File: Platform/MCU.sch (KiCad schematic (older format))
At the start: 34 parts, among them J10 Conn_01x05, J11 Aardvark Header SPI, J12 Aardvark Header I2C, J13 ESP8266_CONN, J14 Aardvark Header I2C, J4 Conn_01x05, J6 Debug Hdr, J7 Conn_01x05, U3 ATSAMD21E16B-M

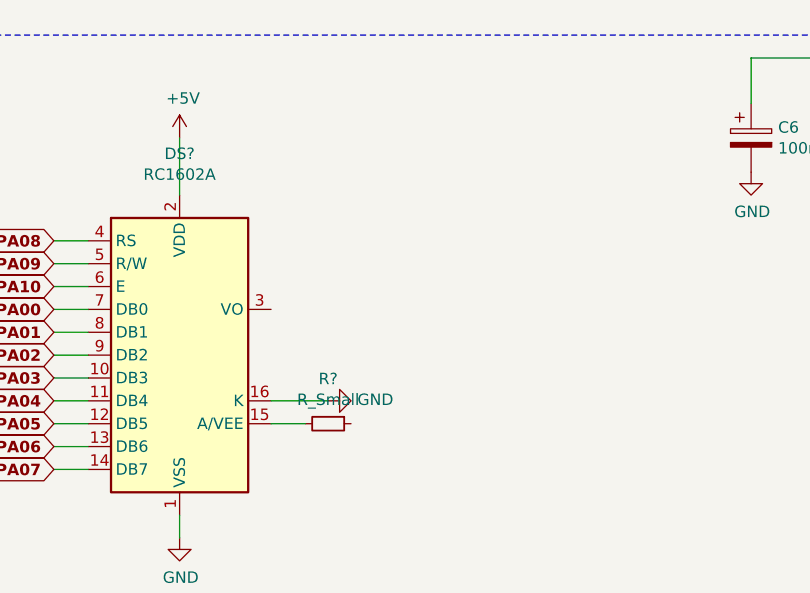
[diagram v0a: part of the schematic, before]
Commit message: Updated the schematic.
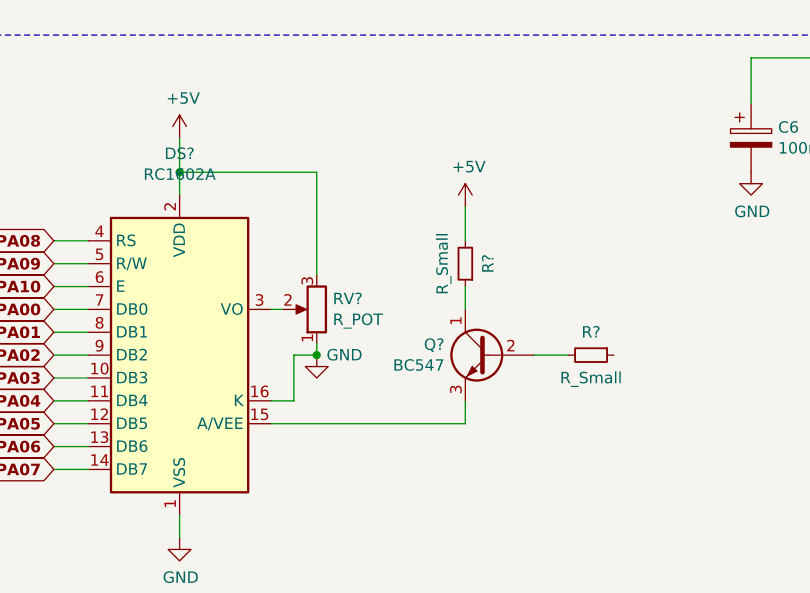
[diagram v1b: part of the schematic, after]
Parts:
- added Q?: BC547, Package_TO_SOT_THT:TO-92_Inline, symbol Transistor_BJT:BC547
- added R?: R_Small, symbol Device:R_Small
- added RV?: R_POT, symbol Device:R_POT
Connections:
- net +5V: now also R?.2, RV?.3
- net GND: now also RV?.1
- net at DS?.15 (A/VEE): now also Q?.3 (E); no longer R?.2
- net at DS?.3 (VO): now also RV?.2
- new net: Q?.1 (C), R?.1
- new net: Q?.2 (B), R?.2
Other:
- moved on the sheet: R?
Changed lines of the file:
@@
 	1750 3150 1750 3050
 Wire Wire Line
-	1750 1400 1750 1650
+	1750 1400 1750 1550
 Text GLabel 1200 1850 0    50   BiDi ~ 10
 PA08
@@
 L Device:R_Small R?
 U 1 1 6020D43B
-P 2400 2650
-F 0 "R?" V 2204 2650 50  0000 C CNN
-F 1 "R_Small" V 2295 2650 50  0000 C CNN
-F 2 "" H 2400 2650 50  0001 C CNN
-F 3 "~" H 2400 2650 50  0001 C CNN
-	1    2400 2650
+P 3550 2350
+F 0 "R?" V 3450 2350 50  0000 C CNN
+F 1 "R_Small" V 3650 2350 50  0000 C CNN
+F 2 "" H 3550 2350 50  0001 C CNN
+F 3 "~" H 3550 2350 50  0001 C CNN
+	1    3550 2350
 	0    1    1    0
 $EndComp
@@
 L power:GND #PWR?
 U 1 1 60207B70
-P 2400 2550
-F 0 "#PWR?" H 2400 2300 50  0001 C CNN
-F 1 "GND" V 2405 2422 50  0000 R CNN
-F 2 "" H 2400 2550 50  0001 C CNN
-F 3 "" H 2400 2550 50  0001 C CNN
-	1    2400 2550
-	0    -1   -1   0
+P 2350 2350
+F 0 "#PWR?" H 2350 2100 50  0001 C CNN
+F 1 "GND" H 2550 2350 50  0000 R CNN
+F 2 "" H 2350 2350 50  0001 C CNN
+F 3 "" H 2350 2350 50  0001 C CNN
+	1    2350 2350
+	1    0    0    -1
+$EndComp
+$Comp
+L power:+5V #PWR?
+U 1 1 601A2CF8
+P 3000 1700
+F 0 "#PWR?" H 3000 1550 50  0001 C CNN
+F 1 "+5V" H 3015 1873 50  0000 C CNN
+F 2 "" H 3000 1700 50  0001 C CNN
+F 3 "" H 3000 1700 50  0001 C CNN
+	1    3000 1700
+	1    0    0    -1
+$EndComp
+$Comp
+L Device:R_POT RV?
+U 1 1 601A87D3
+P 2350 2150
+F 0 "RV?" H 2280 2104 50  0000 R CNN
+F 1 "R_POT" H 2280 2195 50  0000 R CNN
+F 2 "" H 2350 2150 50  0001 C CNN
+F 3 "~" H 2350 2150 50  0001 C CNN
+	1    2350 2150
+	-1   0    0    1
 $EndComp
 Wire Wire Line
-	2150 2550 2400 2550
+	2200 2150 2150 2150
 Wire Wire Line
-	2300 2650 2150 2650
+	2350 2000 2350 1550
+Wire Wire Line
+	2350 1550 1750 1550
+Connection ~ 1750 1550
+Wire Wire Line
+	1750 1550 1750 1650
+Wire Wire Line
+	2350 2350 2350 2300
+Wire Wire Line
+	2350 2350 2250 2350
+Wire Wire Line
+	2250 2350 2250 2550
+Wire Wire Line
+	2250 2550 2150 2550
+Connection ~ 2350 2350
+$Comp
+L Transistor_BJT:BC547 Q?
+U 1 1 601C0547
+P 3100 2350
+F 0 "Q?" H 3291 2396 50  0000 L CNN
+F 1 "BC547" H 3291 2305 50  0000 L CNN
+F 2 "Package_TO_SOT_THT:TO-92_Inline" H 3300 2275 50  0001 L CIN
+F 3 "https://www.onsemi.com/pub/Collateral/BC550-D.pdf" H 3100 2350 50  0001 L CNN
+	1    3100 2350
+	-1   0    0    -1
+$EndComp
+$Comp
+L Device:R_Small R?
+U 1 1 601C3595
+P 3000 1950
+F 0 "R?" V 2900 1950 50  0000 C CNN
+F 1 "R_Small" V 3100 1950 50  0000 C CNN
+F 2 "" H 3000 1950 50  0001 C CNN
+F 3 "~" H 3000 1950 50  0001 C CNN
+	1    3000 1950
+	-1   0    0    1
+$EndComp
+Wire Wire Line
+	3000 2550 3000 2650
+Wire Wire Line
+	3000 2650 2150 2650
+Wire Wire Line
+	3000 2150 3000 2050
+Wire Wire Line
+	3000 1700 3000 1850
+Wire Wire Line
+	3300 2350 3450 2350
 $EndSCHEMATC
